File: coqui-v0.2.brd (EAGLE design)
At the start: 71 x 18.3 mm, 21 parts, among them IC3 MCP73831, IC4 MCP1700-33, J1 AYZ0202, X1 USBSMD

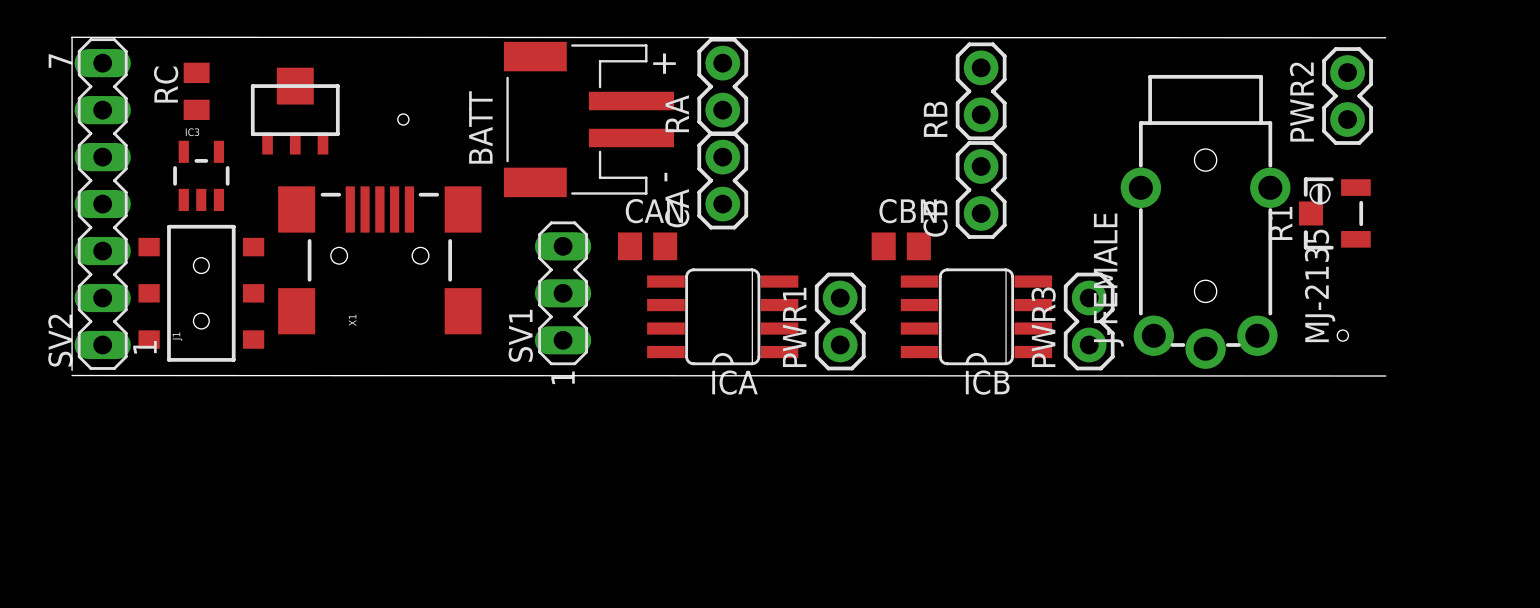
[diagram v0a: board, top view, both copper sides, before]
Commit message: update
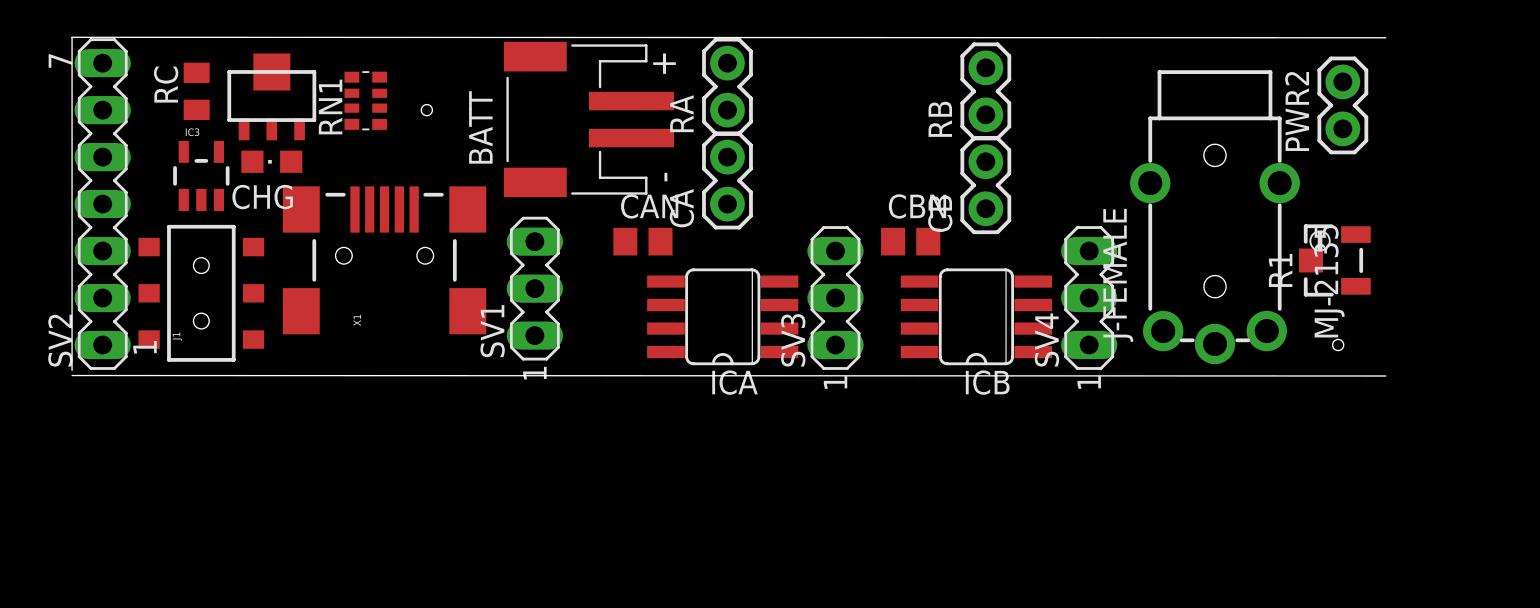
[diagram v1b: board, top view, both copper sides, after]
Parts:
- removed PWR1, PWR3: M02PTH, SparkFun-Connectors:1X02
- added CHG: 0805, led:CHIPLED_0805
- added RN1: (no value), resistor-dil:EXB38V
- added SV3, SV4: (no value), con-lstb:MA03-1
- moved R1 2.54 mm to (67.8, 14.7)
- moved SV1 1.55 mm to (24.6, 13.2)
- moved IC4 1.48 mm to (10.4, 23.6)
- moved PWR2 0.57 mm to (68.3, 21.8)
- moved CBN 0.57 mm to (45.0, 15.7)
- moved J-FEMALE 0.57 mm to (57.9, 10.4)
- moved CAN 0.36 mm to (30.5, 15.7)
- moved CB 0.36 mm to (49.0, 17.5)
- moved X1 0.25 mm to (16.5, 15.0)
- moved CA 0.25 mm to (35.1, 17.8)
- moved RA 0.25 mm to (35.1, 22.9)
- moved RB 0.25 mm to (49.0, 22.6)
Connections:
- new net N$5: CHG.C
- new net N$8: CHG.A, RN1.1
- new net VBUS1: RN1.8

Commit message: update
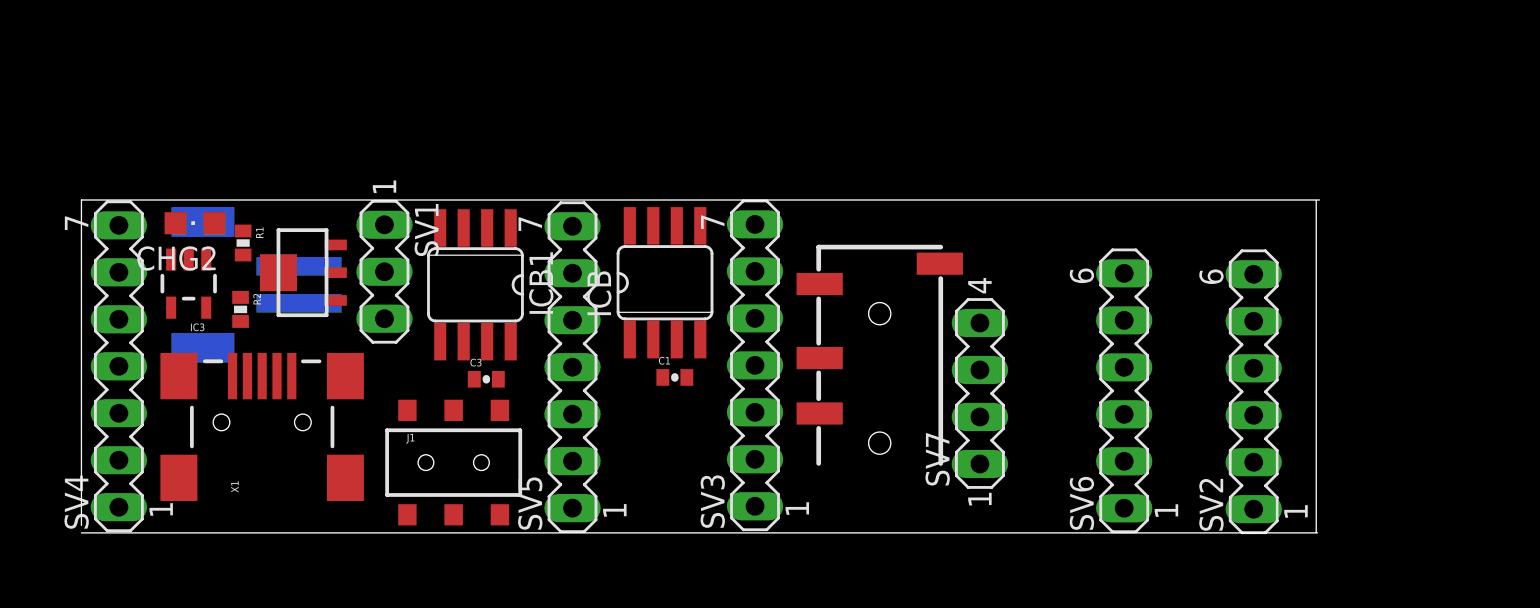
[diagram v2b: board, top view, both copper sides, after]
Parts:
- removed CA, CB, PWR2, RA, RB: M02PTH, SparkFun-Connectors:1X02
- removed CAN, CBN: 0.01uF, rcl:C0805@1
- removed CHG: 0805, led:CHIPLED_0805
- removed ICA: LM555D, adafruit:SO08
- removed J-FEMALE: MJ-2135, iPhoneSoftModem:MJ-2135
- removed RC: 22K, adafruit2013:R0805
- removed RN1: (no value), resistor-dil:EXB38V
- added C1, C3: .01uF, SparkFun:0402-CAP
- added CHG2: 0805, led:CHIPLED_0805
- added ICB1: LM555D, adafruit:SO08
- added JP2: AUDIO-JACK3, SparkFun-Connectors:AUDIO-JACK-TRRS-SMD
- added R2: 22k, SparkFun:0402-RES
- added SV5: (no value), con-lstb:MA07-1
- added SV6: (no value), con-lstb:MA06-1
- added SV7: (no value), con-lstb:MA04-1
- R1: value (none) -> 10k; device pot:3223W -> SparkFun:0402-RES
- SV2: device con-lstb:MA07-1 -> con-lstb:MA06-1
- SV3, SV4: device con-lstb:MA03-1 -> con-lstb:MA07-1
- moved SV2 63.1 mm to (63.5, 7.63)
- moved R1 59.0 mm to (8.86, 15.7), turned to 270 degrees
- moved SV4 52.6 mm to (2.15, 9.01)
- moved BATT 20.1 mm to (8.19, 13.4), flipped to the bottom, turned to 270 degrees
- moved ICB 16.9 mm to (31.7, 13.5), turned to 0 degrees
- moved J1 16.4 mm to (20.2, 3.80), turned to 0 degrees
- moved X1 11.2 mm to (9.89, 5.98)
- moved IC4 9.70 mm to (12.1, 14.1), turned to 90 degrees
- moved SV1 8.18 mm to (16.5, 14.1), turned to 270 degrees
- moved IC3 5.87 mm to (5.92, 13.5), turned to 180 degrees
- moved SV3 5.67 mm to (36.5, 9.06)
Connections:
- removed net BOUT: ICA.3, RB.2
- removed net N$15: CBN.2, ICA.5
- removed net N$16: CB.2, ICA.2, ICA.6, RB.1
- removed net N$6: J-FEMALE.4
- removed net N$8: CHG.A, RN1.1
- removed net VBIN: ICA.4, ICA.8
- removed net VBUS1: RN1.8
- new net AOUT1: ICB1.3, SV5.3, SV5.7
- new net N$1: ICB1.2, ICB1.6, SV5.5, SV5.6
- new net N$2: C1.2, ICB1.5
- new net N$4: CHG2.A, R1.1
- new net RING1: JP2.RING1
- new net RING2: JP2.RING2
- new net SLEEVE: JP2.EARTH
- new net TIP: JP2.TIP
- new net VAIN1: ICB1.4, ICB1.8, SV5.2
- net AOUT: now also SV3.3, SV3.7; no longer RA.2
- net GND: now also C1.1, C3.1, ICB1.1, R2.1, SV1.2, SV1.3, SV3.1, SV3.4, SV5.1, SV5.4; no longer CA.1, CAN.1, CB.1, CBN.1, ICA.1, RC.1
- net N$11: now also SV3.5, SV3.6; no longer CA.2, RA.1
- net N$14: now also C3.2; no longer CAN.2
- net N$3: now also R2.2; no longer RC.2
- net N$5: now also CHG2.C, IC3.1; no longer CHG.C
- net VAIN: now also SV3.2
- net VBUS: now also R1.2
- net VCC: now also SV1.1
- net VDD: now also J1.6
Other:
- board size 71 x 18.3 mm -> 66.9 x 18 mm

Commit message: update
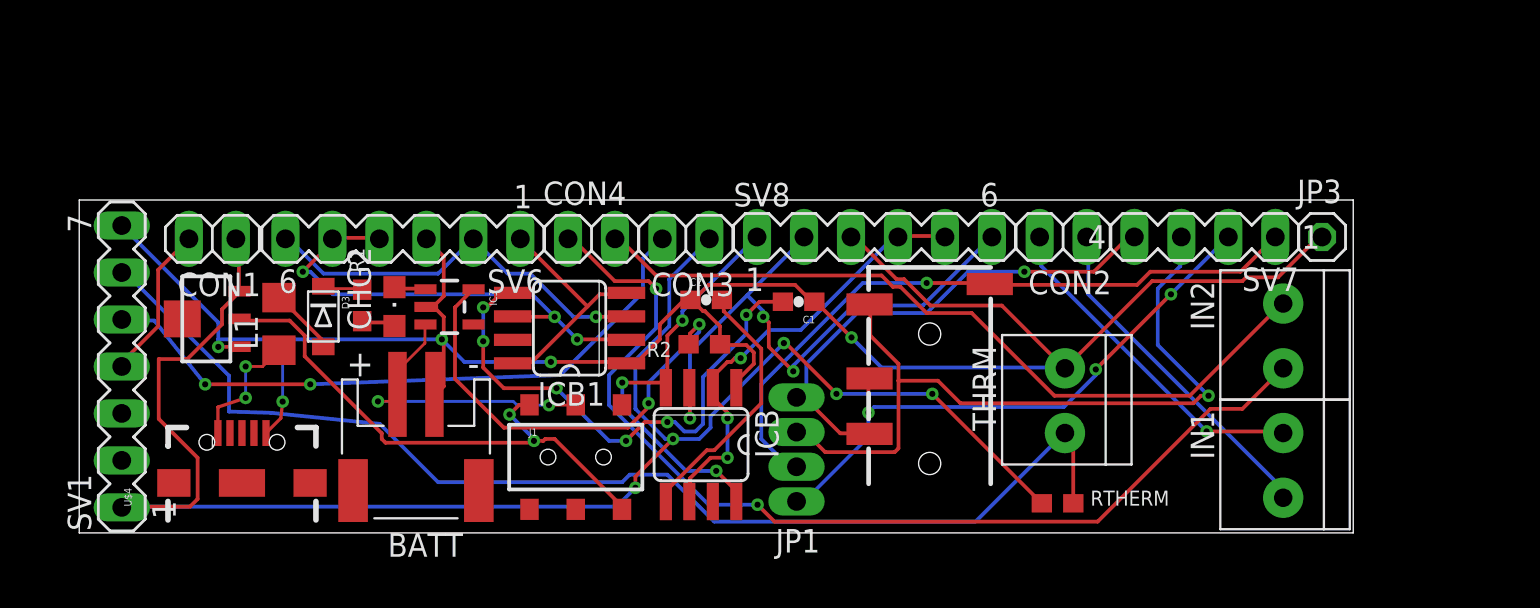
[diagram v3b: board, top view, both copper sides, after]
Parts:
- removed C3: .01uF, SparkFun:0402-CAP
- removed SV2: (no value), con-lstb:MA06-1
- removed SV3, SV4, SV5: (no value), con-lstb:MA07-1
- removed X1: USBSMD, SparkFun:USB-MINIB
- added C2: 0.1uF, SparkFun:0603-CAP
- added CON1, CON2, CON3, CON4: (no value), pinhead:1X02
- added D3: SCHOTTKY, adafruit:SOD-123FL
- added IN1, IN2, THRM: 1X2-3.5MM, adafruit:1X2-3.5MM
- added JP1: (no value), trrs-dwb:1X04/90
- added JP3: (no value), pinhead:1X01
- added L1: 500mA, adafruit:R1206
- added RTHERM: 10k, microbuilder:0603-NO
- added SV8: (no value), con-lstb:MA06-1
- added U$4: (no value), Testing:USB-AB-MICRO-SMD_V02_BOSS
- C1: value .01uF -> 0.1uF; device SparkFun:0402-CAP -> SparkFun:0603-CAP
- R1, R2: device SparkFun:0402-RES -> microbuilder:0603-NO
- SV1: device con-lstb:MA03-1 -> con-lstb:MA07-1
- moved SV6 39.9 mm to (17.5, 15.9), turned to 180 degrees
- moved R2 25.1 mm to (33.8, 10.2), turned to 180 degrees
- moved SV1 15.1 mm to (2.30, 9.00), turned to 90 degrees
- moved SV7 14.8 mm to (60.9, 16.0), turned to 180 degrees
- moved IC3 14.2 mm to (20.0, 12.2), turned to 270 degrees
- moved BATT 13.9 mm to (18.2, 3.79), flipped to the top, turned to 180 degrees
- moved CHG2 11.7 mm to (17.0, 12.2), turned to 0 degrees
- moved ICB 8.97 mm to (33.6, 4.77), turned to 180 degrees
- moved C1 7.85 mm to (38.9, 12.5), turned to 180 degrees
- moved R1 7.27 mm to (15.3, 12.3), turned to 90 degrees
- moved J1 6.61 mm to (26.8, 4.10)
- moved IC4 5.77 mm to (6.87, 11.6)
- moved ICB1 5.60 mm to (26.5, 11.1), turned to 90 degrees
- moved JP2 2.92 mm to (46.0, 2.15)
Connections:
- removed net RING1: JP2.RING1
- removed net RING2: JP2.RING2
- removed net SLEEVE: JP2.EARTH
- removed net TIP: JP2.TIP
- new net N$10: CON2.2, IN1.1
- new net N$12: L1.1, U$4.VBUS1
- new net N$13: D3.A, L1.2
- new net N$15: CON2.1, IN1.2
- new net N$16: CON4.2, IN2.1
- new net N$17: CON4.1, IN2.2
- new net N$18: CON1.2, SV1.4
- new net N$19: CON3.2, SV1.5
- new net N$6: JP1.4, JP2.EARTH, SV7.1
- new net N$7: JP1.3, JP2.RING1, SV7.2
- new net N$8: JP1.2, JP2.TIP, SV7.3
- new net N$9: JP1.1, JP2.RING2, SV7.4
- new net THRM: RTHERM.2, SV1.6, THRM.2
- new net VIN: IC3.4
- net AOUT: now also SV8.2, SV8.6; no longer SV3.3, SV3.7
- net AOUT1: now also SV6.2, SV6.6; no longer SV5.3, SV5.7
- net GND: now also C2.1, JP3.1, SV1.7, SV6.3, SV8.3, THRM.1, U$4.GND1; no longer C3.1, SV1.2, SV1.3, SV3.1, SV3.4, SV5.1, SV5.4, X1.GND
- net N$1: now also SV6.4, SV6.5; no longer SV5.5, SV5.6
- net N$11: now also SV8.4, SV8.5; no longer SV3.5, SV3.6
- net N$14: now also C2.2; no longer C3.2
- net VAIN: now also SV8.1; no longer SV3.2
- net VAIN1: now also SV6.1; no longer SV5.2
- net VBUS: now also D3.C; no longer IC3.4, X1.VBUS
- net VCC: now also CON1.1, CON3.1, RTHERM.1
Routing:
- net GND: track 0.00 -> 115.2 mm, vias 0 -> 5
- net VCC: track 0.00 -> 93.3 mm, vias 0 -> 5
- net THRM: track 0.00 -> 63.8 mm
- net N$17: track 0.00 -> 55.7 mm, vias 0 -> 2
- net N$8: track 0.00 -> 42.2 mm, vias 0 -> 1
- net N$16: track 0.00 -> 41.7 mm
- net N$6: track 0.00 -> 36.7 mm, vias 0 -> 1
- net N$19: track 0.00 -> 35.1 mm, vias 0 -> 2
- net AOUT: track 0.00 -> 33.1 mm, vias 0 -> 3
- net N$7: track 0.00 -> 32.1 mm, vias 0 -> 3
- net VDD: track 0.00 -> 29.3 mm, vias 0 -> 2
- net N$2: track 0.00 -> 28.6 mm, vias 0 -> 6
- net N$9: track 0.00 -> 27.4 mm, vias 0 -> 1
- net N$1: track 0.00 -> 26.3 mm, vias 0 -> 3
- net N$11: track 0.00 -> 24.2 mm, vias 0 -> 3
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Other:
- board size 66.9 x 18 mm -> 68.9 x 18 mm

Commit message: update
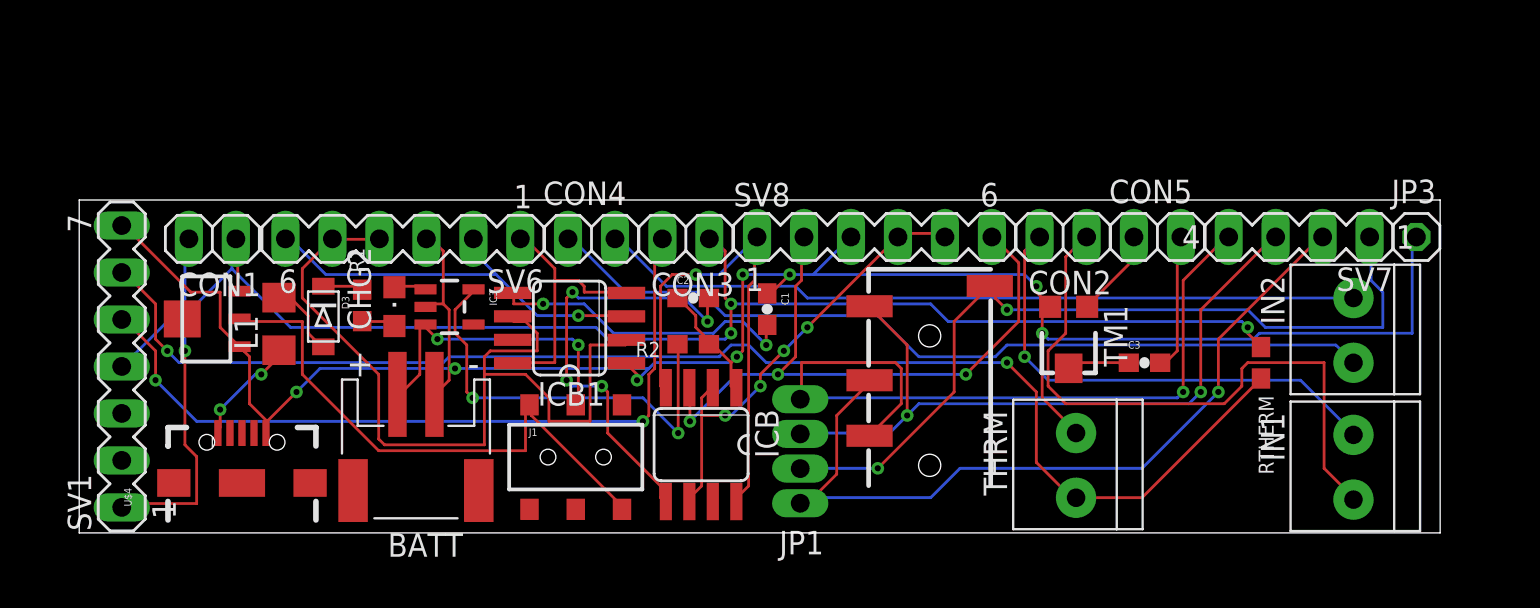
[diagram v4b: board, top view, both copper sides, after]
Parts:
- added C3: 0.1uF, SparkFun:0603-CAP
- added CON5: (no value), pinhead:1X02
- added TM1: (no value), adafruit:TC33X
- moved RTHERM 13.4 mm to (63.9, 9.20), turned to 270 degrees
- moved JP3 5.10 mm to (72.3, 16.0)
- moved SV7 5.10 mm to (66.0, 16.0)
- moved IN2 3.81 mm to (68.9, 10.9)
- moved IN1 3.80 mm to (68.9, 3.50)
- moved THRM 3.55 mm to (53.9, 3.60)
- moved C1 1.75 mm to (37.2, 12.1), turned to 270 degrees
- moved C2 0.71 mm to (33.2, 12.7)
- moved R2 0.60 mm to (33.2, 10.2)
- moved JP1 0.22 mm to (36.7, 4.30)
- moved JP2 0.10 mm to (46.0, 2.05)
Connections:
- new net N$20: CON5.1, TM1.1
- new net N$21: C3.2, CON5.2
- new net N$22: C3.1, TM1.2
- net GND: now also TM1.3
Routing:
- net N$1: track 26.3 -> 46.0 mm, vias 3 -> 0
- net N$15: track 18.5 -> 33.8 mm
- net N$9: track 27.4 -> 42.2 mm
- net N$7: track 32.1 -> 44.5 mm, vias 3 -> 1
- net N$2: track 28.6 -> 16.8 mm, vias 6 -> 2
- net N$17: track 55.7 -> 45.8 mm, vias 2 -> 0
- net N$14: track 14.2 -> 23.9 mm, vias 0 -> 4
- net THRM: track 63.8 -> 73.4 mm, vias 0 -> 2
- net N$10: track 18.4 -> 26.4 mm
- net N$6: track 36.7 -> 44.3 mm, vias 1 -> 2
- net N$21: track 0.00 -> 7.45 mm
- net GND: track 115.2 -> 122.6 mm, vias 5 -> 8
- net N$19: track 35.1 -> 41.7 mm
- net VCC: track 93.3 -> 87.1 mm, vias 5 -> 4
- net N$20: track 0.00 -> 4.84 mm
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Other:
- board size 68.9 x 18 mm -> 73.6 x 18 mm

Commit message: update
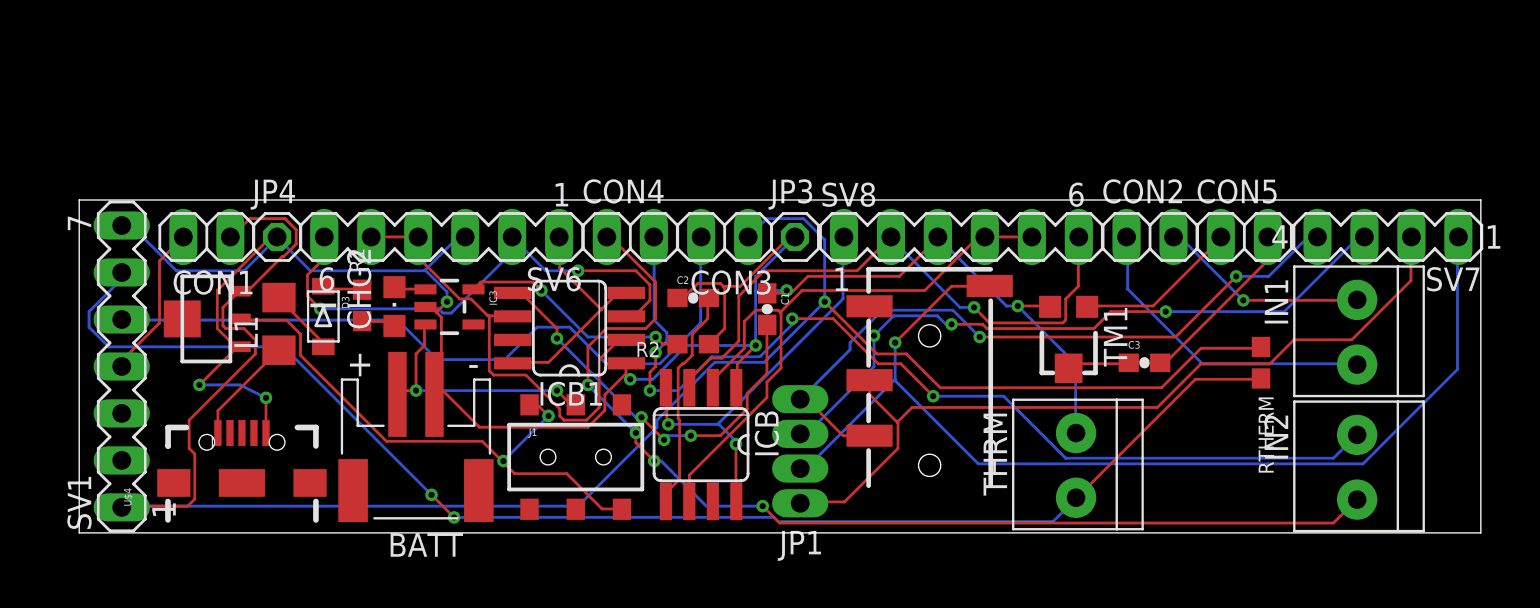
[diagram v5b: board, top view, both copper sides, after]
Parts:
- added JP4: (no value), pinhead:1X01
- moved JP3 33.6 mm to (38.7, 16.0)
- moved IN2 7.40 mm to (69.1, 3.50)
- moved IN1 7.30 mm to (69.1, 10.8)
- moved SV7 4.80 mm to (70.8, 16.0)
- moved CON5 4.70 mm to (63.0, 16.0)
- moved SV8 4.70 mm to (47.7, 16.0)
- moved CON2 4.70 mm to (57.9, 16.0), turned to 0 degrees
- moved CON3 2.10 mm to (34.9, 16.0)
- moved CON4 2.10 mm to (29.8, 16.0)
- moved SV6 2.10 mm to (19.6, 16.0)
- moved CON1 0.32 mm to (6.90, 16.0)
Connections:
- net GND: now also JP4.1
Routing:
- net N$1: track 46.0 -> 25.1 mm
- net VCC: track 87.1 -> 105.4 mm, vias 4 -> 1
- net N$15: track 33.8 -> 16.9 mm
- net N$10: track 26.4 -> 11.4 mm
- net N$6: track 44.3 -> 57.1 mm, vias 2 -> 1
- net N$14: track 23.9 -> 12.1 mm, vias 4 -> 0
- net N$17: track 45.8 -> 57.5 mm, vias 0 -> 4
- net N$16: track 41.2 -> 52.6 mm, vias 0 -> 4
- net N$3: track 23.4 -> 12.6 mm
- net N$11: track 24.4 -> 34.1 mm, vias 4 -> 0
- net AOUT1: track 22.7 -> 28.5 mm, vias 1 -> 2
- net N$2: track 16.8 -> 22.0 mm, vias 2 -> 4
- net GND: track 122.6 -> 117.6 mm, vias 8 -> 7
- net N$9: track 42.2 -> 37.6 mm, vias 1 -> 2
- net VAIN: track 26.8 -> 22.3 mm, vias 1 -> 2
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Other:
- board size 73.6 x 18 mm -> 75.8 x 18 mm
